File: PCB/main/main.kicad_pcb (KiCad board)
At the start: 2 copper layers, 19 parts, among them IC1 EL5171ISZ-T7, J1 Conn_01x33_Female, J2 Conn_01x33_Female, J3 Conn_01x33_Female, J4 Conn_01x33_Female

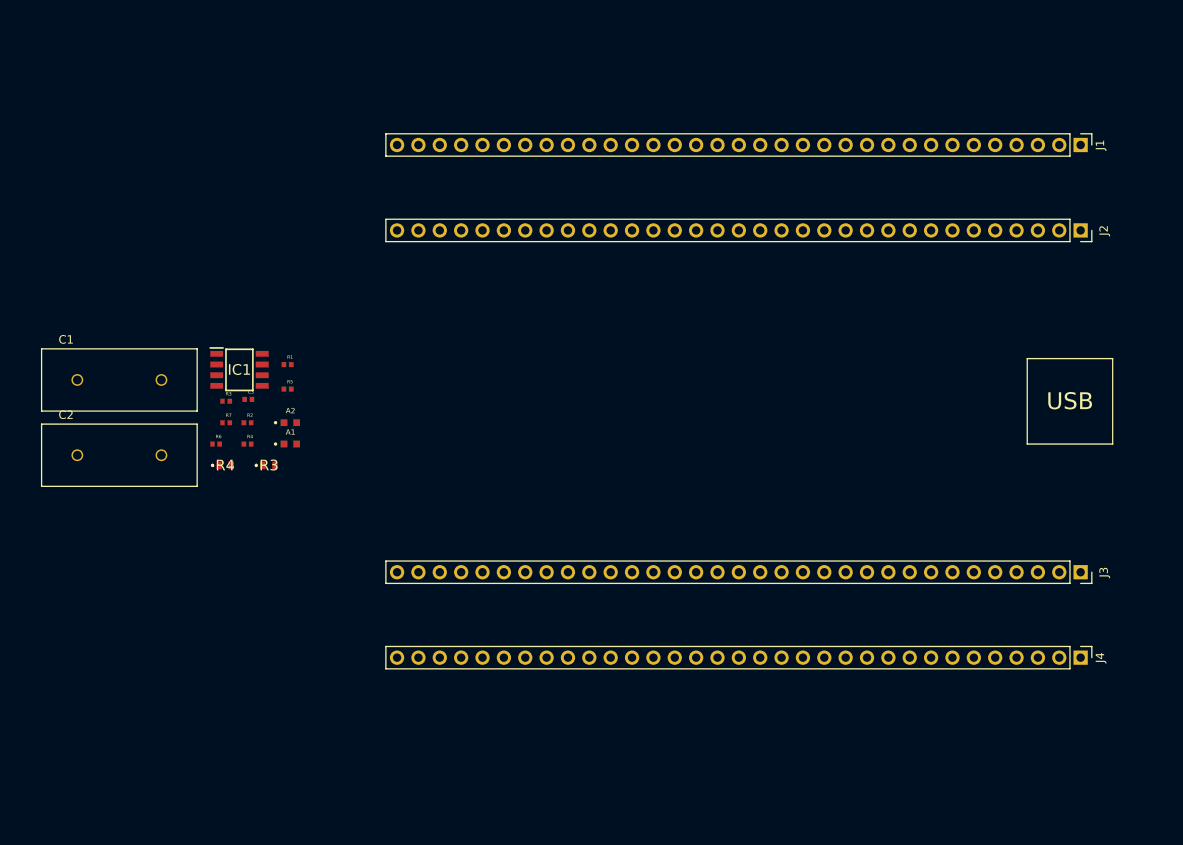
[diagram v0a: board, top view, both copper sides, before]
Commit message: updated stuff
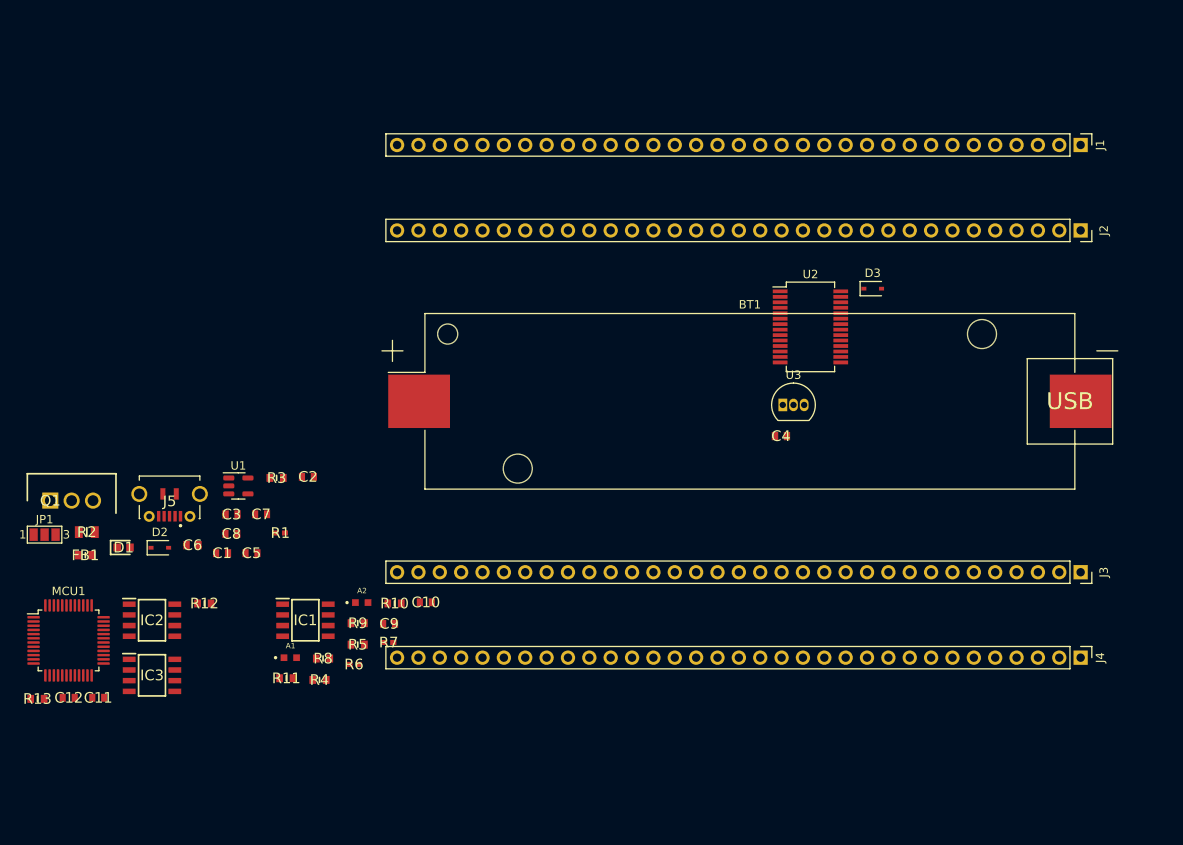
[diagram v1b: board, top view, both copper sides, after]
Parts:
- removed the R3 at (83.8, 104.1)
- removed the R3 at (78.7, 96.5)
- removed the R4 at (78.6, 104.1)
- removed the R4 at (81.3, 101.6)
- added BT1: 3.7V, Battery:BatteryHolder_Keystone_1042_1x18650, F.Cu at (141.0, 96.5)
- added C10: CL10A105KB8NNNC, SamacSys_Parts:CAPC1608X90N, F.Cu at (102.5, 120.4)
- added C11: CL10A335KP8NNNC, SamacSys_Parts:CAPC1608X90N, F.Cu at (63.5, 131.8)
- added C12: CL10A335KP8NNNC, SamacSys_Parts:CAPC1608X90N, F.Cu at (60.0, 131.8)
- added C4: CL10A475KA8NQNC, SamacSys_Parts_Microcontroller:CAPC1608X95N, F.Cu at (144.7, 100.7)
- added C5: 100nF, SamacSys_Parts:CAPC1608X90N, F.Cu at (81.8, 114.6)
- added C6: CL10A475KA8NQNC, SamacSys_Parts_Microcontroller:CAPC1608X95N, F.Cu at (74.7, 113.6)
- added C7: 1uF, SamacSys_Parts:CAPC1608X90N, F.Cu at (82.9, 110.0)
- added C8: 1uF, SamacSys_Parts:CAPC1608X90N, F.Cu at (79.4, 112.3)
- added C9: CL10A105KB8NNNC, SamacSys_Parts:CAPC1608X90N, F.Cu at (98.1, 123.0)
- added D1: LED, SamacSys_Parts:LEDC1608X70N, F.Cu at (66.5, 113.9)
- added D2: BAT60J, Diode_SMD:D_SOD-323, F.Cu at (70.8, 113.9)
- added D3: BAT60J, Diode_SMD:D_SOD-323, F.Cu at (155.6, 83.1)
- added FB1: Ferrite_Bead, SamacSys_Parts:BEADC1608X95N, F.Cu at (62.0, 114.8)
- added IC2: LM358DT, SamacSys_Parts:SOIC127P600X175-8N, F.Cu at (69.9, 122.5)
- added IC3: AT24C256C-SSHL-T, SamacSys_Parts:SOIC127P600X175-8N, F.Cu at (69.9, 129.1)
- added J5: USB_B_Micro, SamacSys_Parts:MICROXNJ, F.Cu at (72.0, 105.4)
- added JP1: Jumper_3_Open, Jumper:SolderJumper-3_P1.3mm_Open_Pad1.0x1.5mm_NumberLabels, F.Cu at (57.1, 112.4)
- added MCU1: STM32F030C8Tx, Package_QFP:LQFP-48_7x7mm_P0.5mm, F.Cu at (60.0, 125.0)
- added Q1: IRF9540NPbF, SamacSys_Parts_Power:TO254P469X1042X1967-3P, F.Cu at (57.8, 108.3)
- added R10: RC0603FR-071KL, SamacSys_Parts:RESC1608X55N, F.Cu at (98.8, 120.5)
- added R11: RC0603FR-071KL, SamacSys_Parts:RESC1608X55N, F.Cu at (85.9, 129.4)
- added R12: RC0603FR-071KL, SamacSys_Parts:RESC1608X55N, F.Cu at (76.1, 120.5)
- added R13: RC0603FR-071KL, SamacSys_Parts:RESC1608X55N, F.Cu at (56.3, 131.9)
- added R3: 10k, SamacSys_Parts:RESC1608X55N, F.Cu at (84.7, 105.6)
- added R4: RC0603FR-071KL, SamacSys_Parts:RESC1608X55N, F.Cu at (89.8, 129.7)
- added R8: RC0603FR-071KL, SamacSys_Parts:RESC1608X55N, F.Cu at (90.3, 127.1)
- added R9: RC0603FR-071KL, SamacSys_Parts:RESC1608X55N, F.Cu at (94.4, 122.9)
- added U1: MCP73831-2-OT, Package_TO_SOT_SMD:SOT-23-5, F.Cu at (80.2, 106.6)
- added U2: FT232RL, Package_SO:SSOP-28_5.3x10.2mm_P0.65mm, F.Cu at (148.2, 87.7)
- added U3: MCP1700-3302E_TO92, Package_TO_SOT_THT:TO-92_Inline, F.Cu at (144.9, 97.0)
- A1, A2: footprint footprints:XDCR_ALS-PT19-315C_L177_TR8 -> SamacSys_Parts:XDCR_ALS-PT19-315C_L177_TR8
- C1: value ECQE2105KFB -> 10nF; footprint footprints:CAPRR1000W80L1850T740H2000 -> SamacSys_Parts:CAPC1608X90N
- C2: value ECQE2105KFB -> 100nF; footprint footprints:CAPRR1000W80L1850T740H2000 -> SamacSys_Parts:CAPC1608X90N
- C3: value GRM1555C1H5R1BA01D -> CL10A475KA8NQNC; footprint footprints:CAPC1005X55N -> SamacSys_Parts_Microcontroller:CAPC1608X95N
- IC1: value EL5171ISZ-T7 -> LM358DT; footprint footprints:SOIC127P600X175-8N -> SamacSys_Parts:SOIC127P600X175-8N
- R1: value AC0402FR-07536KL -> 2k; footprint footprints:RESC1005X37N -> SamacSys_Parts:RESC1005X35N
- R2: value AC0402FR-07536KL -> RC0805FR-07470RL; footprint footprints:RESC1005X37N -> SamacSys_Parts_Microcontroller:RESC2012X60N
- R5: value AC0402FR-07536KL -> RC0603FR-071KL; footprint footprints:RESC1005X37N -> SamacSys_Parts:RESC1608X55N
- R6, R7: value AC0402JR-0750RL -> AC0402FR-07536KL; footprint footprints:RESC1005X37N -> SamacSys_Parts:RESC1005X37N
- moved R7 32.5 mm to (98.1, 125.2)
- moved R5 31.5 mm to (94.4, 125.5)
- moved R6 30.9 mm to (93.9, 127.8)
- moved IC1 30.8 mm to (88.2, 122.5)
- moved A1 25.4 mm to (86.4, 127.0)
- moved C1 23.9 mm to (78.2, 114.6)
- moved R2 23.1 mm to (62.2, 112.1)
- moved A2 23.0 mm to (94.9, 120.5)
- moved C2 22.6 mm to (88.5, 105.5)
- moved R1 20.0 mm to (85.2, 112.2)
- moved C3 13.8 mm to (79.4, 110.0)
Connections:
- A1 pad 1: Vsupply -> +3v3
- A1 pad 2: Sensor Signal -> Vout1
- A2 pad 1: Vsupply -> +3v3
- A2 pad 2: Net-(A2-Pad2) -> Vout2
- C1 pad 1: GND -> Earth
- C1 pad 2: Sensor Signal -> +5V
- C2 pad 1: GND -> Earth
- C2 pad 2: Net-(A2-Pad2) -> Net-(C2-Pad2)
- C3 pad 1: Net-(C3-Pad1) -> Earth
- C3 pad 2: GND -> +5V
- IC1 pad 1: Net-(IC1-Pad1) -> Vdiff
- IC1 pad 2: Net-(A2-Pad2) -> IN1-
- IC1 pad 3: Sensor Signal -> IN1+
- IC1 pad 4: Net-(IC1-Pad4) -> -3v3
- IC1 pad 5: Net-(C3-Pad1) -> GND
- IC1 pad 6: +5v -> IN2-
- IC1 pad 7: -5v -> -3v3
- IC1 pad 8: Vdiff -> +3v3
- R1 pad 1: GND -> Net-(R1-Pad1)
- R1 pad 2: Sensor Signal -> Earth
- R2 pad 1: GND -> Net-(D1-Pad1)
- R2 pad 2: Net-(A2-Pad2) -> Net-(R2-Pad2)
- R5 pad 1: Net-(IC1-Pad1) -> GND
- R5 pad 2: Net-(IC1-Pad4) -> IN2-
- R6 pad 1: GND -> Vout1
- R6 pad 2: Net-(A2-Pad2) -> GND
- R7 pad 1: GND -> Vout2
- R7 pad 2: Sensor Signal -> GND

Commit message: git main schematics updated
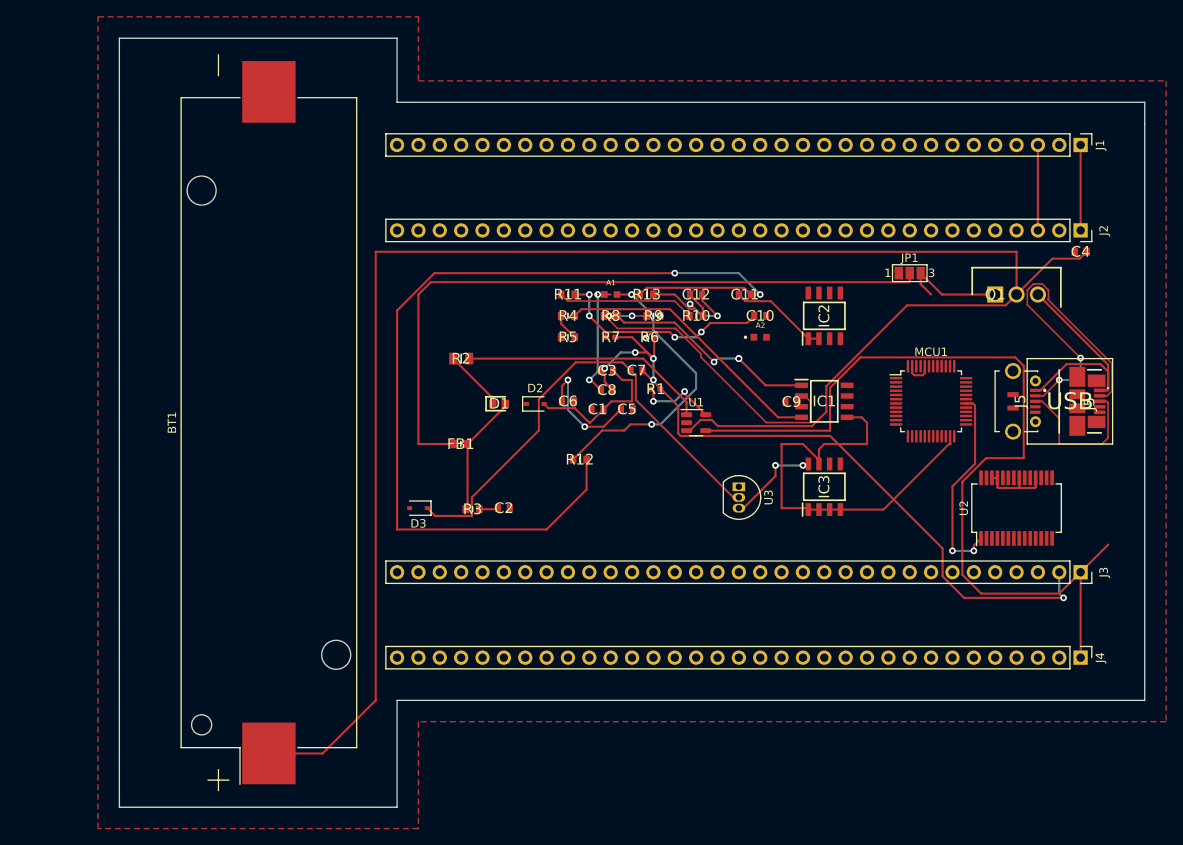
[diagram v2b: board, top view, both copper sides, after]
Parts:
- added J5: 47346-0001, SamacSys_Parts_Power:47346-0001, F.Cu at (177.8, 96.5)
- moved Q1 115.0 mm to (170.2, 83.8)
- moved JP1 107.5 mm to (160.0, 81.3)
- moved MCU1 106.4 mm to (162.6, 96.5)
- moved J5 98.6 mm to (170.2, 96.5), turned to 90 degrees
- moved C11 90.6 mm to (140.4, 83.8)
- moved C12 88.7 mm to (134.6, 83.8)
- moved IC2 87.8 mm to (149.9, 86.4), turned to 90 degrees
- moved R13 86.9 mm to (128.7, 83.8)
- moved IC3 83.0 mm to (149.9, 106.7), turned to 90 degrees
- moved IC1 67.0 mm to (149.9, 96.5)
- moved D3 60.0 mm to (101.6, 109.2), turned to 180 degrees
- moved A1 57.6 mm to (124.5, 83.8)
- moved BT1 57.2 mm to (83.8, 99.1), turned to 90 degrees
- moved A2 56.9 mm to (142.2, 88.9)
- moved R11 56.6 mm to (119.4, 83.8)
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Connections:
- BT1 pad 2: Earth -> GND
- C1 pad 1: Earth -> GND
- C2 pad 1: Earth -> GND
- C3 pad 1: Earth -> GND
- C4 pad 1: Earth -> GND
- C5 pad 2: Earth -> GND
- C6 pad 2: Earth -> GND
- C7 pad 2: Earth -> GND
- C8 pad 2: Earth -> GND
- R1 pad 2: Earth -> GND
- R3 pad 2: Earth -> GND
- U1 pad 2: Earth -> GND
- U2 pad 18: Earth -> GND
- U2 pad 21: Earth -> GND
- U2 pad 25: Earth -> GND
- U2 pad 26: Earth -> GND
- U2 pad 7: Earth -> GND
- U3 pad 1: Earth -> GND
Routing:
- net Net-(BT1-Pad1): track 0.00 -> 208.7 mm
- net +5V: track 0.00 -> 166.7 mm
- net GND: track 0.00 -> 156.9 mm, vias 0 -> 5
- net Net-(C11-Pad2): track 0.00 -> 115.1 mm, vias 0 -> 2
- net VCC: track 0.00 -> 96.5 mm, vias 0 -> 2
- net Net-(C7-Pad1): track 0.00 -> 56.8 mm
- net /Power/D-: track 0.00 -> 39.5 mm, vias 0 -> 2
- net IN1-: track 0.00 -> 38.7 mm, vias 0 -> 2
- net Vout1: track 0.00 -> 36.5 mm, vias 0 -> 4
- net -3v3: track 0.00 -> 32.6 mm
- net Net-(R2-Pad2): track 0.00 -> 29.5 mm
- net Vout2: track 0.00 -> 26.6 mm, vias 0 -> 4
- net Vdiff: track 0.00 -> 25.6 mm, vias 0 -> 3
- net +3v3: track 0.00 -> 25.2 mm, vias 0 -> 4
- net USART1_TX: track 0.00 -> 23.9 mm, vias 0 -> 2
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- added copper zone on F.Cu, net GND
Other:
- board outline added: 121.9 x 91.4 mm
